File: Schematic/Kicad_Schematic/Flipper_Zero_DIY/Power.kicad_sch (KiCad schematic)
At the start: 81 parts, among them x10 Connector 3P

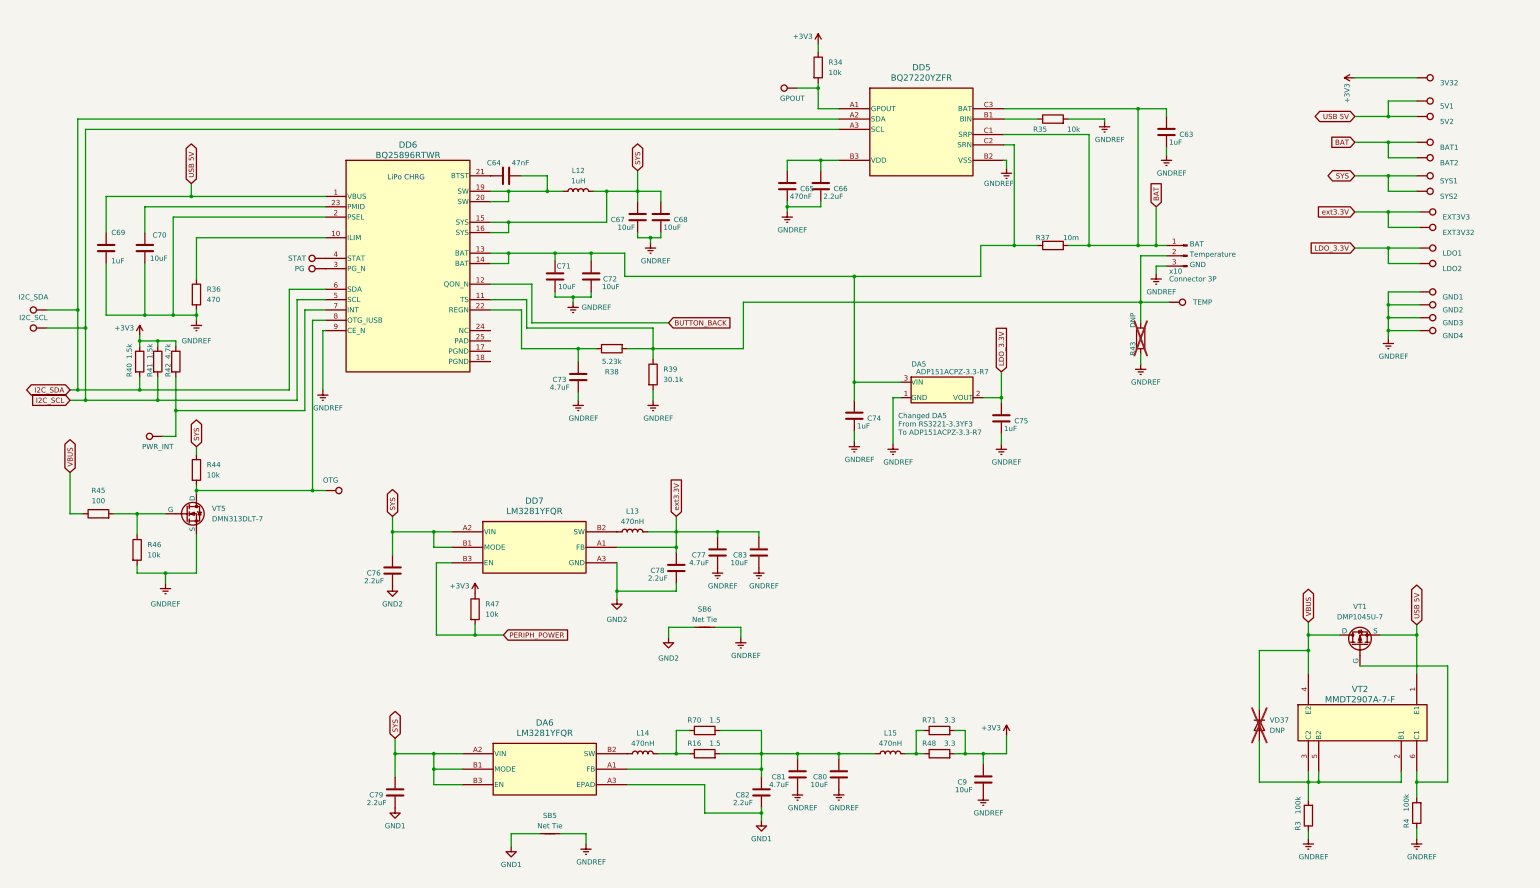
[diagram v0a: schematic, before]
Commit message: added all changes to the changelog
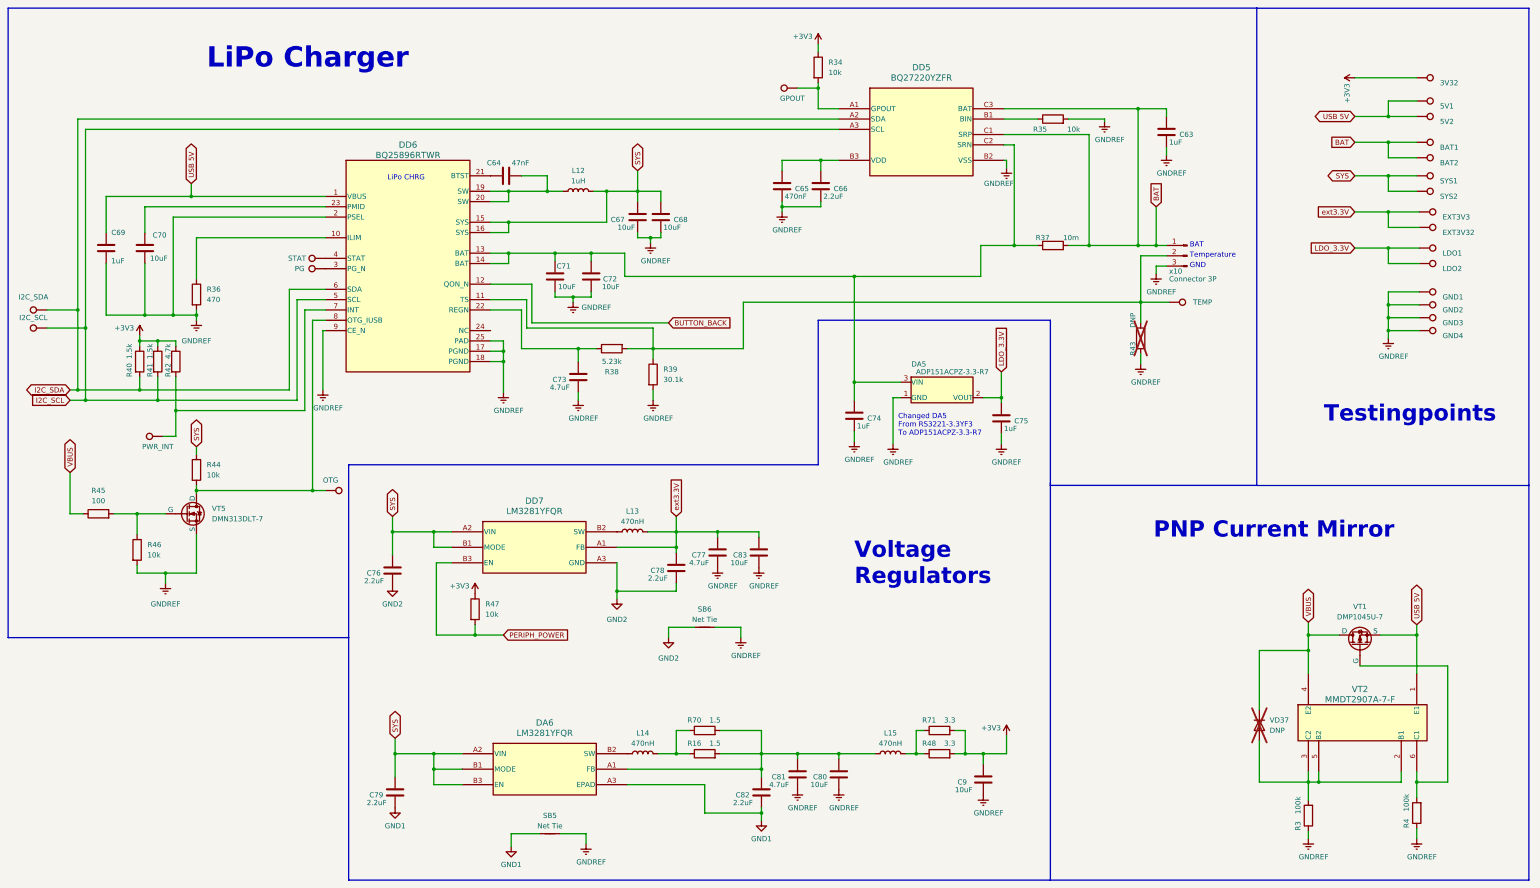
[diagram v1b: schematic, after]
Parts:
- x10: footprint Connector_PinHeader_2.00mm:PinHeader_1x03_P2.00mm_Horizontal -> Connector_PinHeader_2.54mm:PinHeader_1x03_P2.54mm_Horizontal
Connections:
- net GNDREF: now also DD6.17 (PGND), DD6.18 (PGND), DD6.25 (PAD)
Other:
- note added: "LiPo Charger"
- note added: "PNP Current Mirror"
- note added: "Testingpoints"
- note added: "Voltage Regulators"
- moved on the sheet: C65
